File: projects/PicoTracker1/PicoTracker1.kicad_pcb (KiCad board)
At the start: 2 copper layers, 58.4 x 32.4 mm, 32 parts, among them M1 RF4463PRO, M2 UBLOX_NEO-6, U1 ATMEGA328-AU

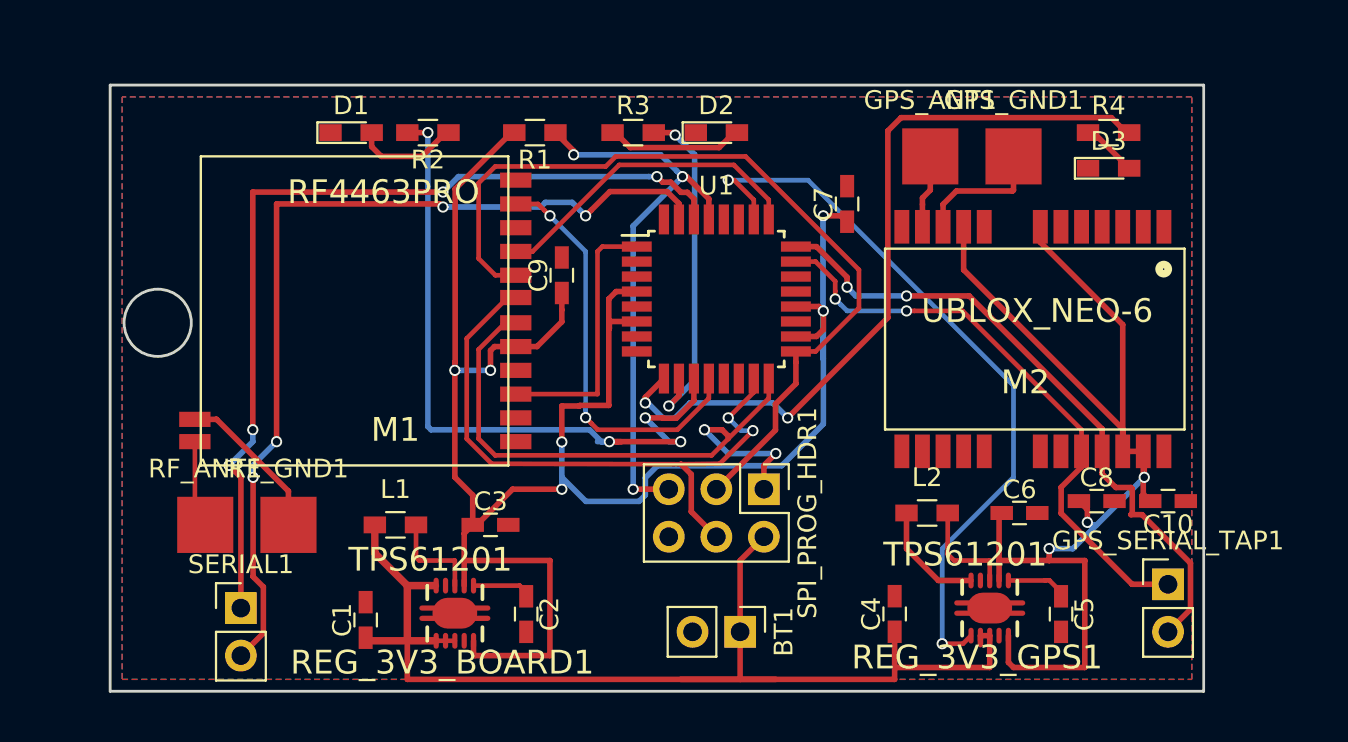
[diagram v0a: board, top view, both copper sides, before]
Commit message: KiCad PicoTracker1 pcb done
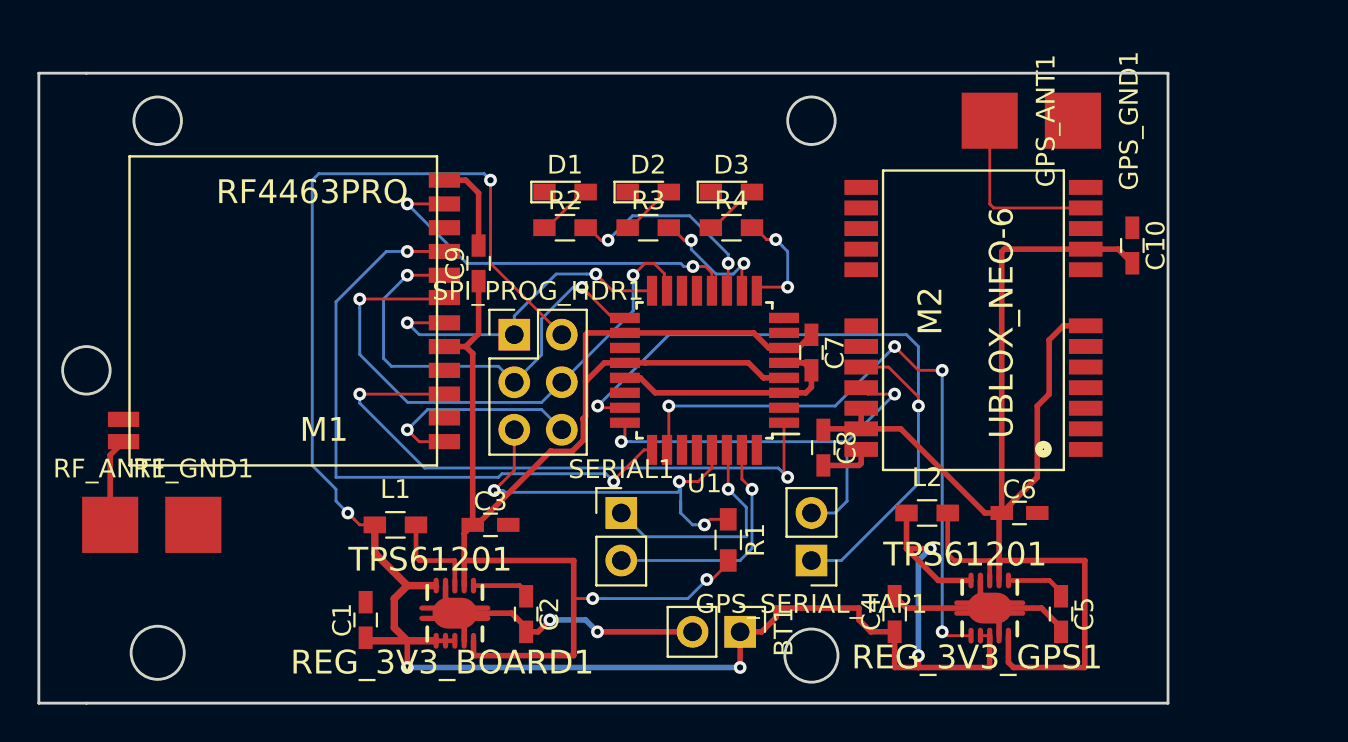
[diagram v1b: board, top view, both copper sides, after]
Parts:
- moved R1 24.1 mm to (208.9, 189.4), turned to 270 degrees
- moved SERIAL1 20.9 mm to (203.2, 188.0)
- moved R4 20.8 mm to (209.1, 172.7)
- moved D3 20.2 mm to (209.1, 170.8)
- moved GPS_SERIAL_TAP1 19.1 mm to (213.4, 190.5), turned to 180 degrees
- moved SPI_PROG_HDR1 15.7 mm to (197.5, 178.4), turned to 0 degrees
- moved C8 14.9 mm to (214.0, 184.5), turned to 270 degrees
- moved C10 13.8 mm to (230.5, 173.7), turned to 270 degrees
- moved D1 11.9 mm to (200.2, 170.8)
- moved R2 8.91 mm to (200.2, 172.7), turned to 0 degrees
- moved C7 8.17 mm to (213.4, 179.4), turned to 270 degrees
- moved R3 5.14 mm to (204.6, 172.7)
- moved RF_ANT1 5.08 mm to (175.9, 188.6)
- moved RF_GND1 5.08 mm to (180.3, 188.6)
- moved D2 4.83 mm to (204.6, 170.8)
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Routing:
- net GND: track 15.5 -> 61.6 mm, vias 0 -> 3
- net VBATT: track 72.9 -> 109.9 mm, vias 0 -> 6
- net Net-(SERIAL1-Pad2): track 49.0 -> 12.7 mm, vias 4 -> 1
- net Net-(SERIAL1-Pad1): track 48.5 -> 12.3 mm, vias 4 -> 1
- net Net-(R4-Pad2): track 41.4 -> 6.06 mm
- net Net-(R2-Pad2): track 38.5 -> 11.3 mm, vias 4 -> 2
- net VCC: track 107.4 -> 81.8 mm, vias 6 -> 2
- net SPI_SCK: track 45.3 -> 24.4 mm, vias 0 -> 2
- net RF_SIGNAL: track 14.2 -> 32.5 mm, vias 0 -> 2
- net SPI_SS_RF: track 17.3 -> 34.2 mm, vias 0 -> 2
- net SPI_MISO: track 33.6 -> 17.6 mm
- net Net-(R3-Pad2): track 18.4 -> 7.07 mm
- net GPS_SER_IN: track 34.9 -> 24.0 mm
- net SPI_RESET: track 30.6 -> 22.0 mm
- net GPS_SER_OUT: track 31.7 -> 39.4 mm
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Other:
- board size 58.4 x 32.4 mm -> 60.3 x 33.7 mm
- net class Default: clearance 0.2 -> 0.1524; trace_width 0.25 -> 0.1524; via_dia 0.6 -> 0.6858; via_drill 0.4 -> 0.3302
- rule trace_clearance: 0.2 -> 0.1524
- rule trace_min: 0.2 -> 0.1524
- rule via_min_drill: 0.3 -> 0.3302
- rule via_min_size: 0.4 -> 0.6858
- board text added: "2018-01-29 - PicoTracker1 - Rev 1"
- board text added: "Safe scientific experiment in Ham Radio (APRS) If found, please contact us! Douglas Malnati (KD2KDD) Mark Malnati (KN4IUD) douglas.malnati@gmail.com 201-993-6716"
